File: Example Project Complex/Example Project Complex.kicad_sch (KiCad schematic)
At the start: 0 parts

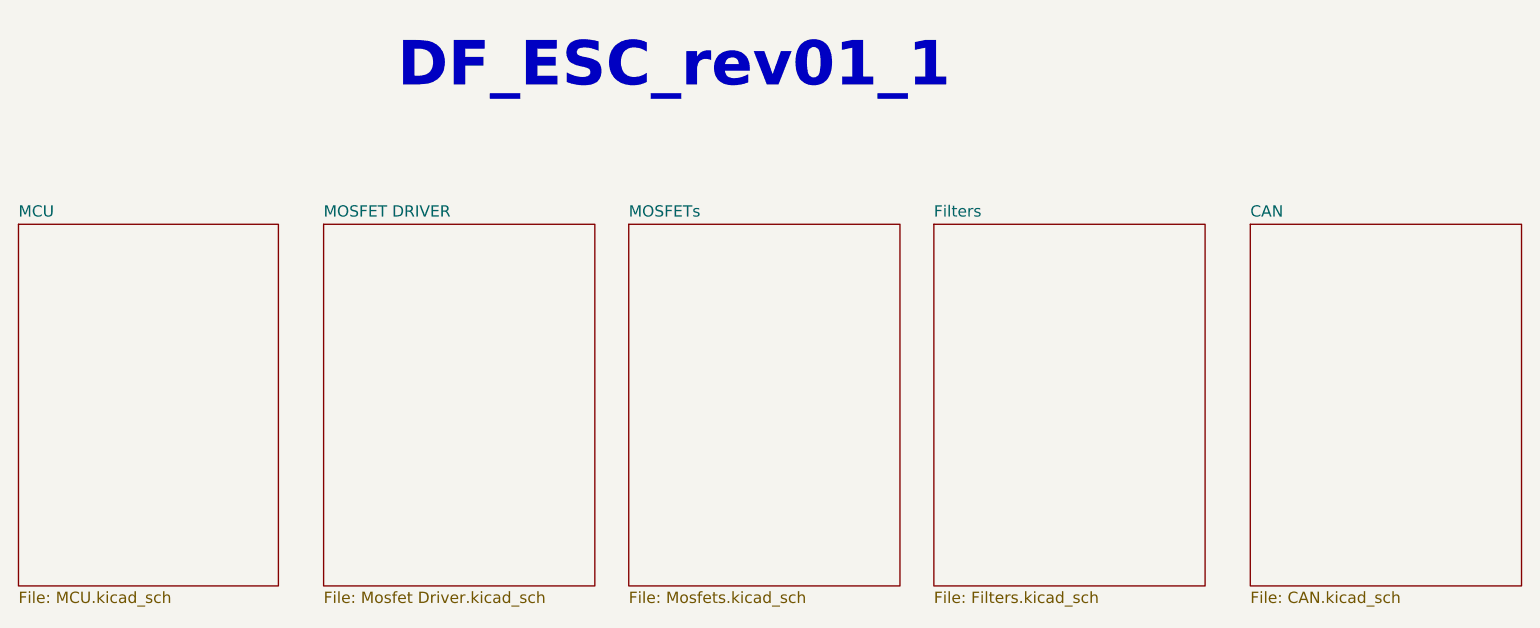
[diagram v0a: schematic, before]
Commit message: dont know updates
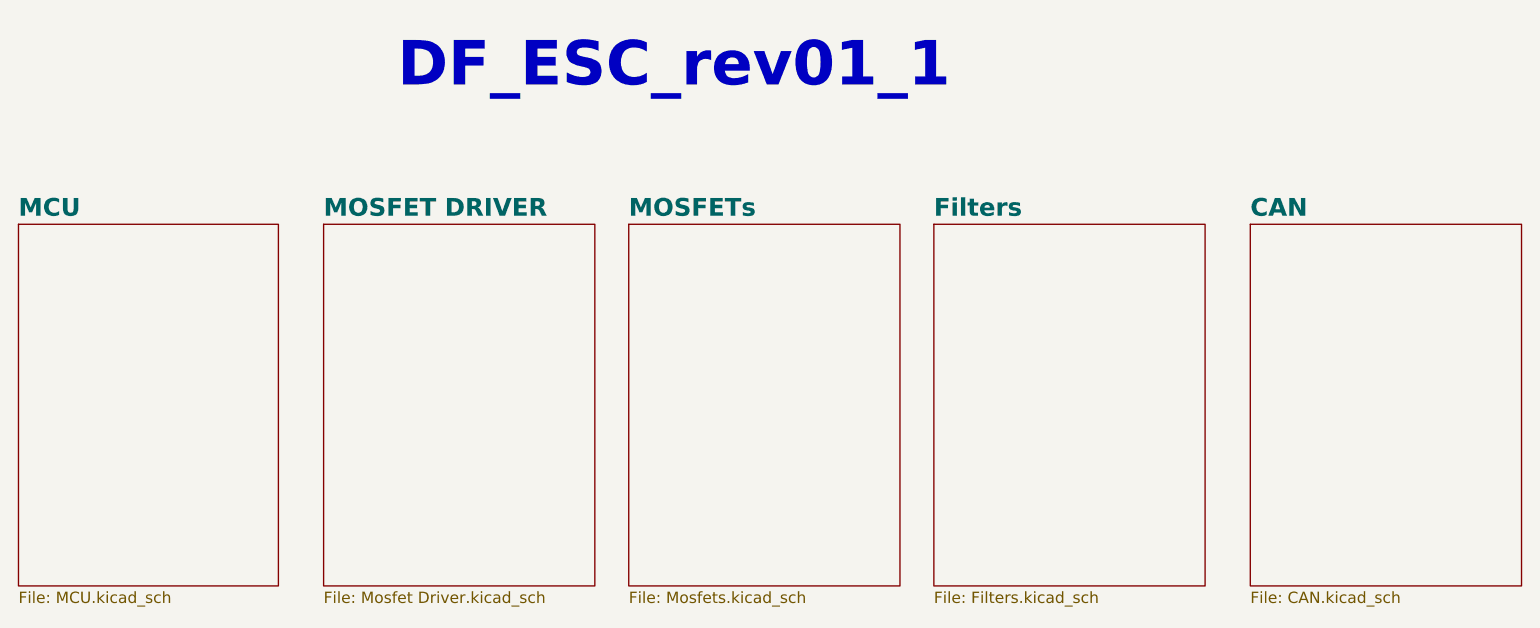
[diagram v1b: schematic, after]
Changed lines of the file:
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@@
 			(effects
 				(font
-					(size 1.27 1.27)
+					(size 2 2)
+					(bold yes)
 				)
 				(justify left bottom)
@@
 			(effects
 				(font
-					(size 1.27 1.27)
+					(size 2 2)
+					(bold yes)
 				)
 				(justify left bottom)
@@
 			(effects
 				(font
-					(size 1.27 1.27)
+					(size 2 2)
+					(bold yes)
 				)
 				(justify left bottom)
@@
 			(effects
 				(font
-					(size 1.27 1.27)
+					(size 2 2)
+					(bold yes)
 				)
 				(justify left bottom)
@@
 			(effects
 				(font
-					(size 1.27 1.27)
+					(size 2 2)
+					(bold yes)
 				)
 				(justify left bottom)
